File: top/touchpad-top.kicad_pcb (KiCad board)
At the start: 2 copper layers, 28.3 x 40 mm, 142 parts, among them P1 CONN_10, P2 CONN_5, U1 IQS572, U4 ESD

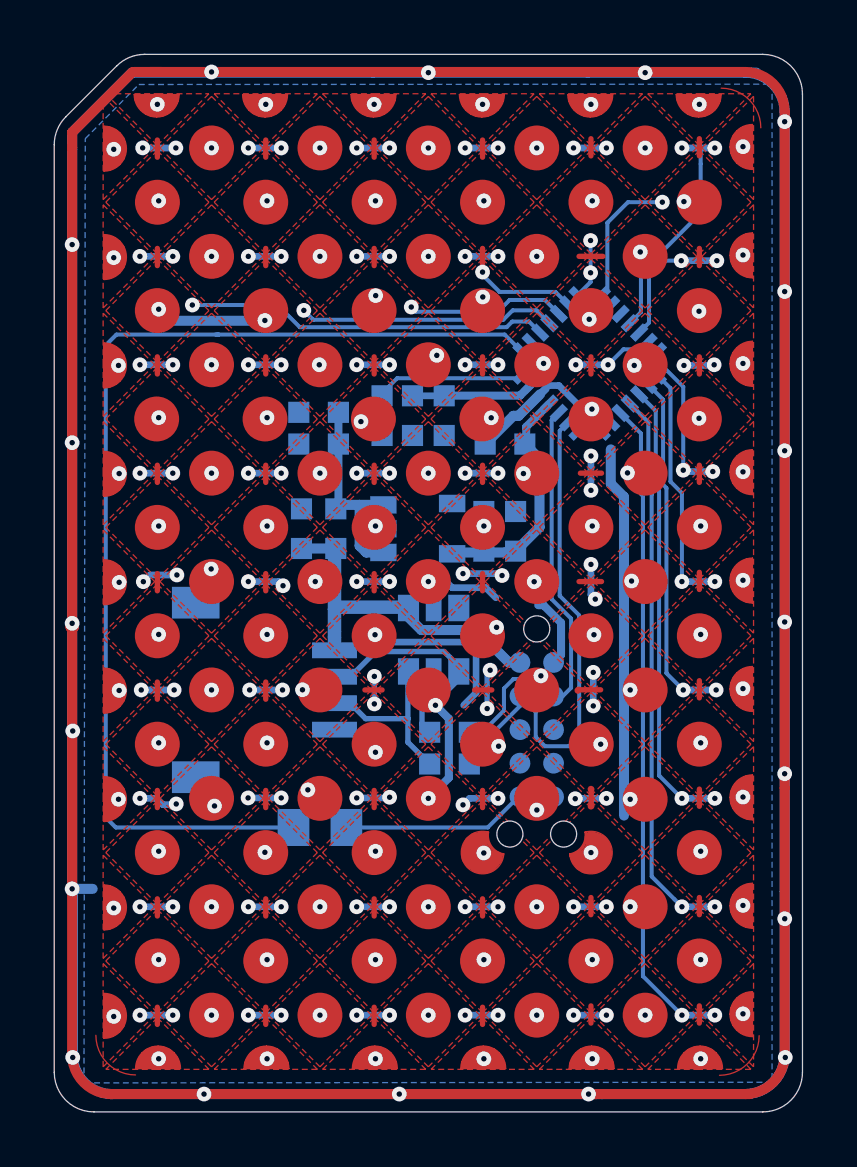
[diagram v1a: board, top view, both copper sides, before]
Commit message: Modified contour.
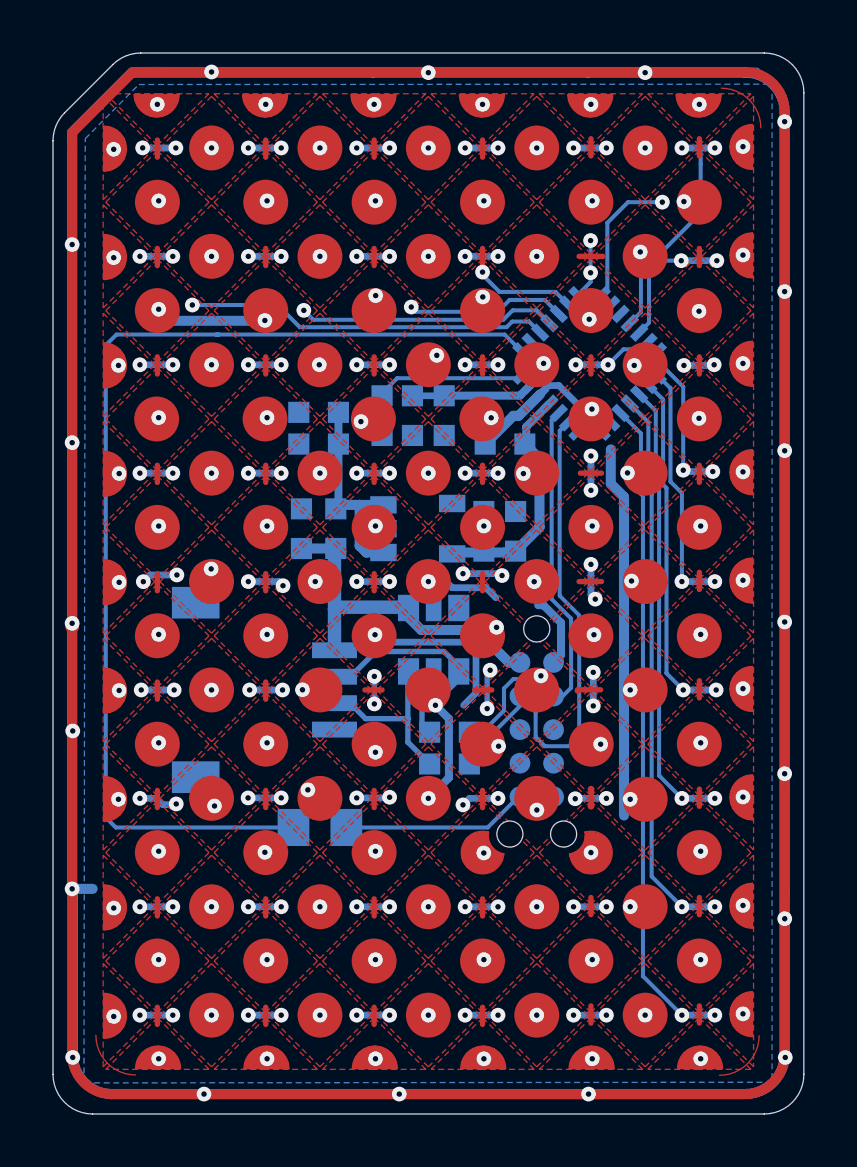
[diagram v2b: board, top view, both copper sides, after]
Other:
- board size 28.3 x 40 mm -> 28.4 x 40.1 mm
